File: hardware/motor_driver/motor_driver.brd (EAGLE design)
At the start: 93.7 x 72.4 mm, 88 parts

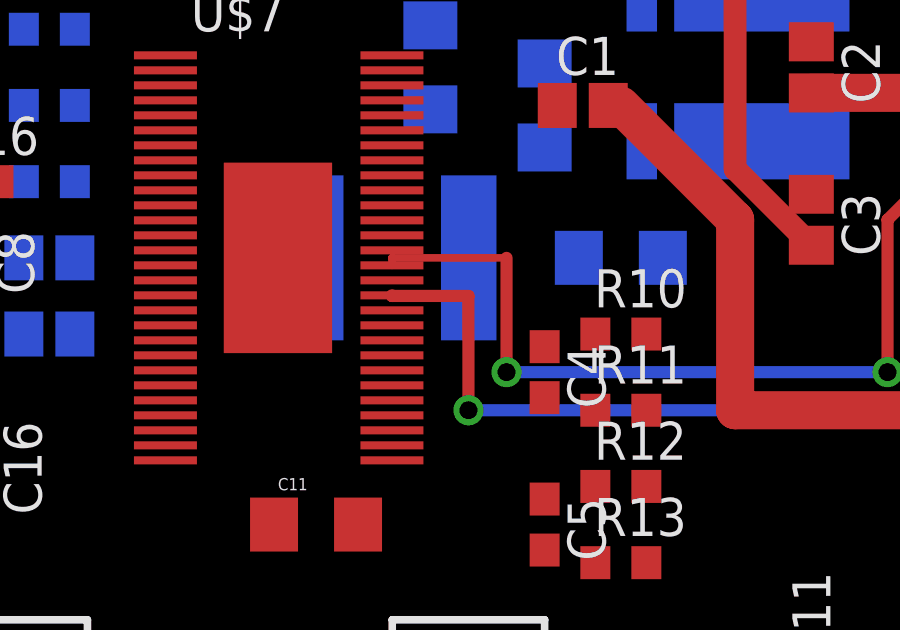
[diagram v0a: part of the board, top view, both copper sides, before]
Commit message: small change
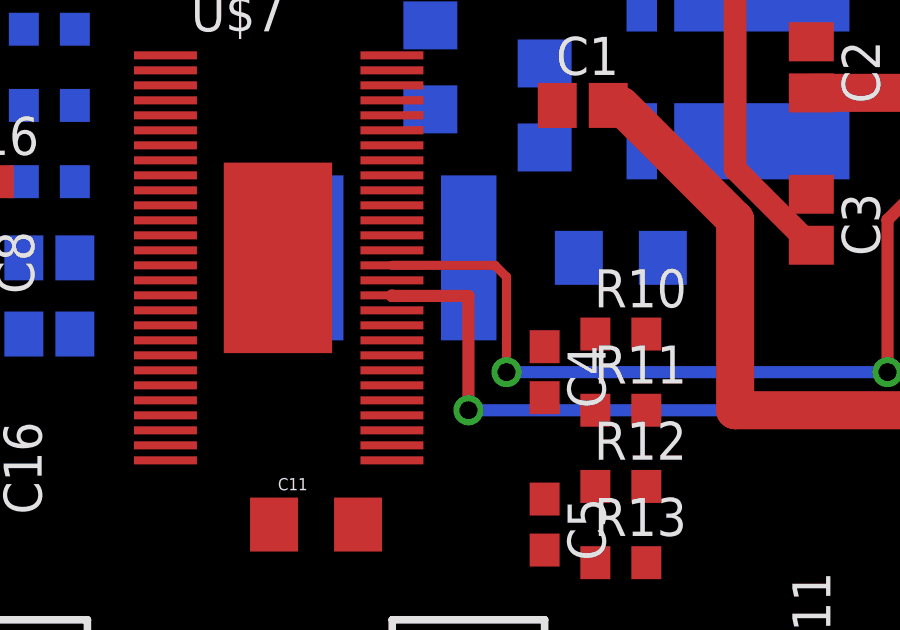
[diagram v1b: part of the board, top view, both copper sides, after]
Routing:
- net GH_B: track 56.1 -> 55.4 mm
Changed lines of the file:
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@@
 <via x="69.85" y="26.67" extent="1-16" drill="0.6" shape="square"/>
 <wire x1="69.85" y1="26.67" x2="69.85" y2="25.4" width="0.4064" layer="1"/>
-<wire x1="60.96" y1="16.51" x2="46.98" y2="18.8" width="0" layer="19" extent="1-16"/>
 <wire x1="69.85" y1="25.4" x2="68.58" y2="25.4" width="0.4064" layer="1"/>
 <wire x1="68.58" y1="25.4" x2="63.5" y2="20.32" width="0.4064" layer="1"/>
@@
 <wire x1="63.5" y1="15.24" x2="50.8" y2="15.24" width="0.4064" layer="16"/>
 <via x="50.8" y="15.24" extent="1-16" drill="0.6" shape="square"/>
-<wire x1="50.8" y1="15.24" x2="50.8" y2="19.05" width="0.4064" layer="1"/>
-<wire x1="50.8" y1="19.05" x2="46.98" y2="19.05" width="0.254" layer="1"/>
-<wire x1="46.98" y1="19.05" x2="46.98" y2="18.8" width="0.254" layer="1"/>
+<wire x1="50.8" y1="15.24" x2="50.8" y2="18.415" width="0.3048" layer="1"/>
+<wire x1="50.8" y1="18.415" x2="50.415" y2="18.8" width="0.3048" layer="1"/>
+<wire x1="50.415" y1="18.8" x2="46.98" y2="18.8" width="0.3048" layer="1"/>
 </signal>
 <signal name="GH_C">
